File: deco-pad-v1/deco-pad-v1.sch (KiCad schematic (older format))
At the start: 84 parts, among them SW1 EC11, SW2 EC11, SW3 EC11, SW4 SW_Push, U1 ATmega32U4-MU, Y1 16MHz

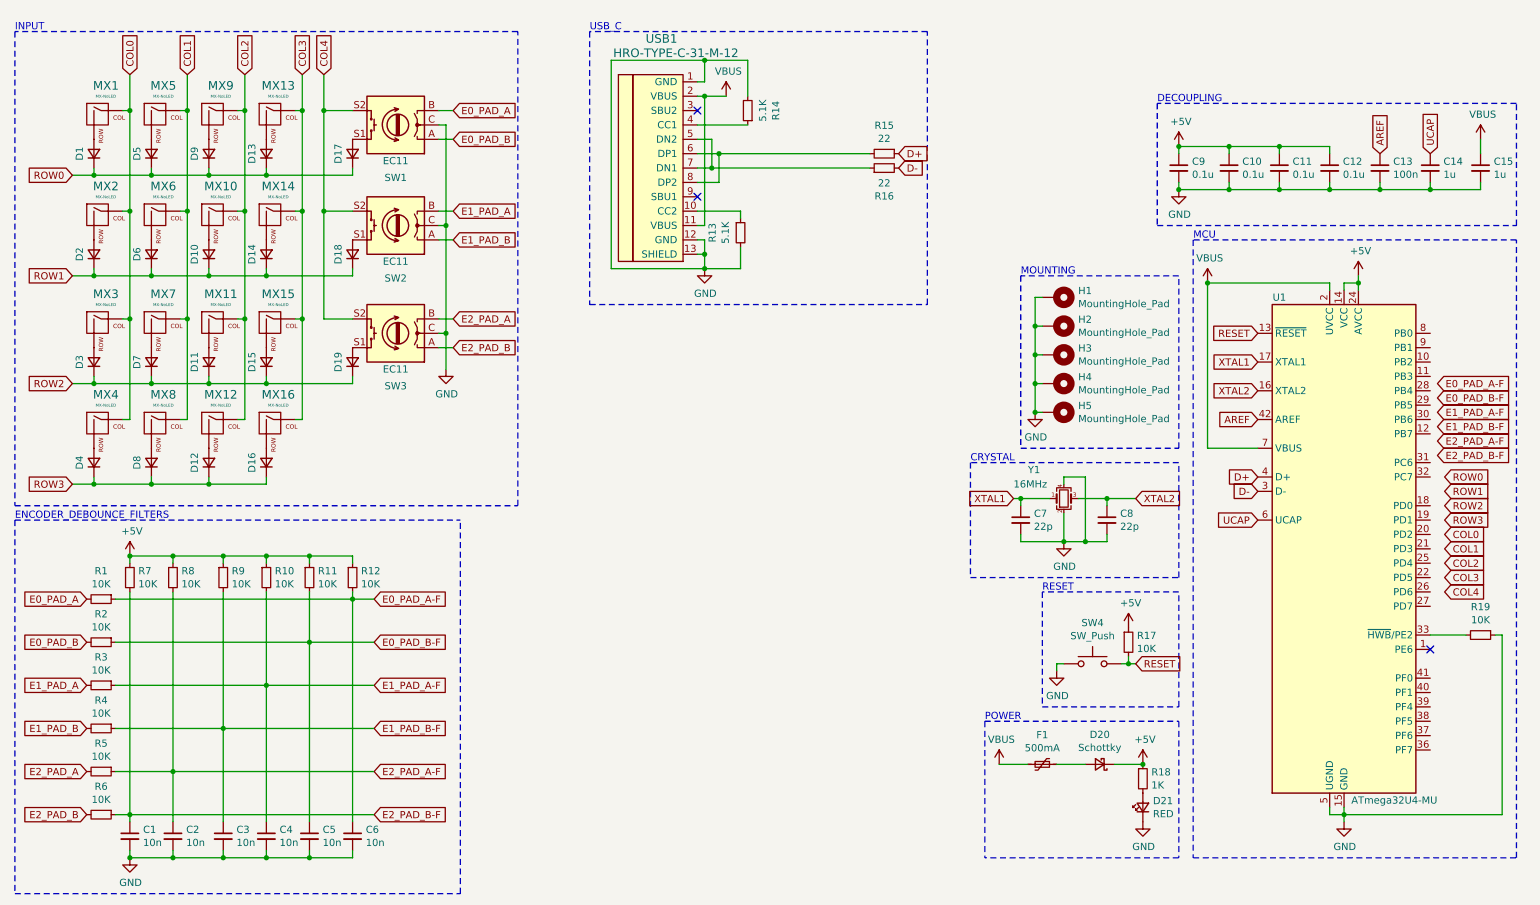
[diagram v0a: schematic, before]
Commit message: [NZ] Schematic and Footprints done.
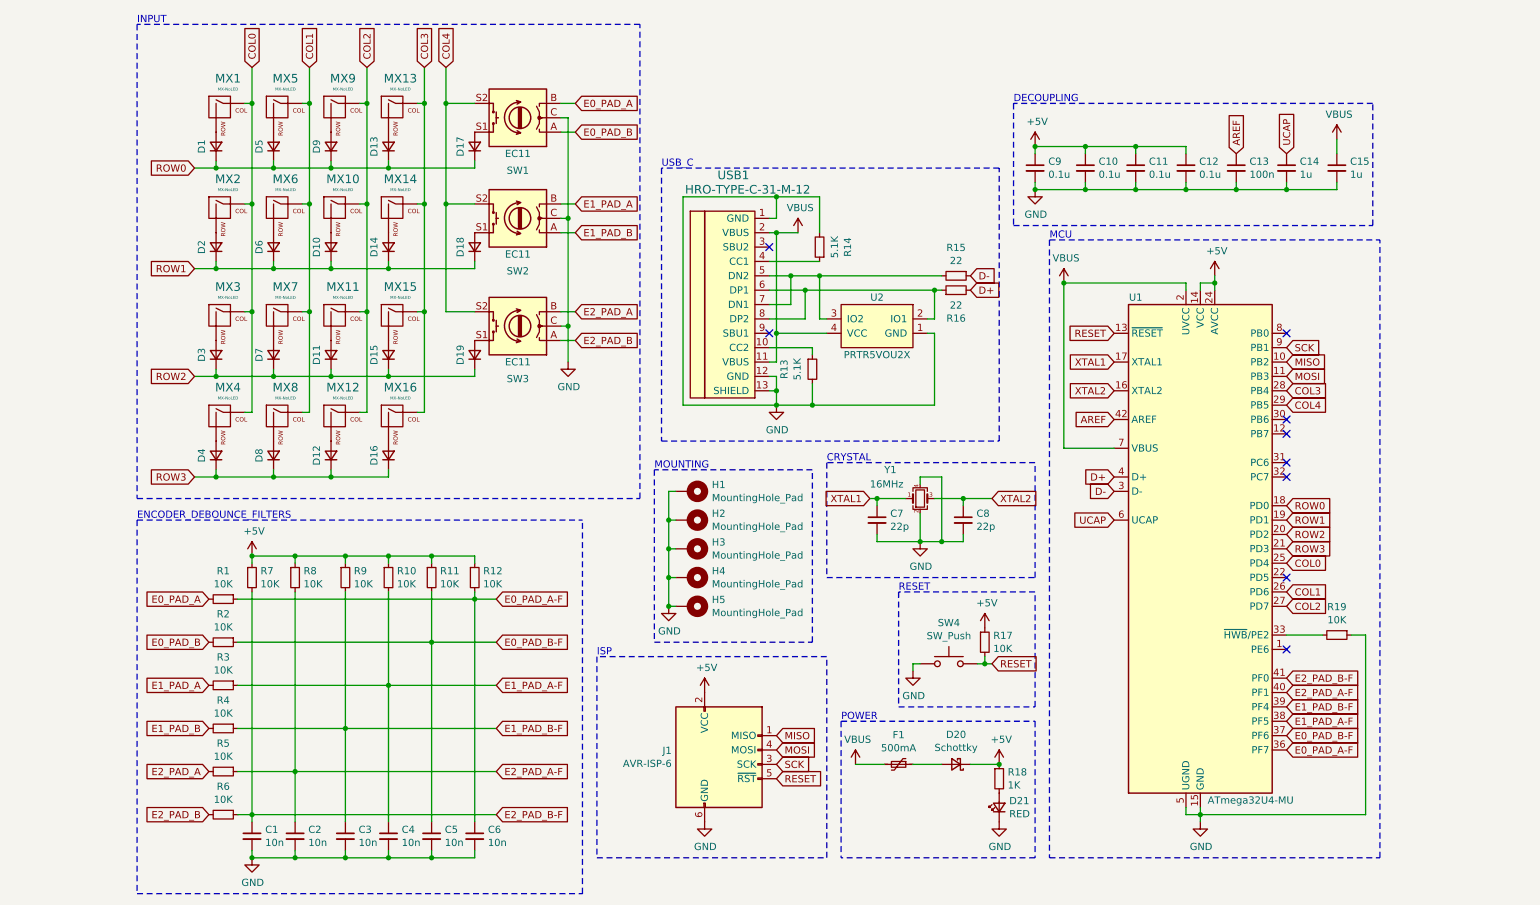
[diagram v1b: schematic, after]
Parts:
- added J1: AVR-ISP-6, Connector_PinSocket_2.54mm:PinSocket_2x03_P2.54mm_Vertical, symbol Connector:AVR-ISP-6
- added U2: PRTR5VOU2X, Nexperia:SOT143B, symbol prtr5vou2x:PRTR5VOU2X
- C1, C10, C11, C12, C13, C14, C2, C3, C4, C5, C6, C7, C8, C9: footprint Capacitor_SMD:C_0603_1608Metric -> Capacitor_SMD:C_0805_2012Metric
- D1, D10, D11, D12, D13, D14, D15, D16, D17, D18, D19, D2, D20, D3, D4, D5, D6, D7, D8, D9: footprint (none) -> Diode_SMD:D_SOD-123
- D21: footprint (none) -> LED_SMD:LED_0805_2012Metric
- F1: footprint (none) -> Fuse:Fuse_1206_3216Metric
- MX1, MX10, MX11, MX12, MX13, MX14, MX15, MX16, MX2, MX3, MX4, MX5, MX6, MX7, MX8, MX9: footprint (none) -> mx-alps-hybrid:MX-1U-NoLED
- R1, R10, R11, R12, R13, R14, R15, R16, R17, R18, R19, R2, R3, R4, R5, R6, R7, R8, R9: footprint (none) -> Resistor_SMD:R_0805_2012Metric
- SW1, SW2, SW3: footprint (none) -> Rotary_Encoder:RotaryEncoder_Alps_EC11E-Switch_Vertical_H20mm
- SW4: footprint (none) -> Button_Switch_SMD:SW_SPST_B3S-1000
- Y1: footprint (none) -> Crystal:Crystal_SMD_3225-4Pin_3.2x2.5mm
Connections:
- net +5V: now also J1.2 (VCC)
- net COL0: now also U1.25 (PD4)
- net COL1: now also U1.26 (PD6)
- net COL2: now also U1.27 (PD7)
- net COL3: now also U1.28 (PB4)
- net COL4: now also U1.29 (PB5)
- net D+: now also R16.2; no longer R15.1
- net D-: now also R15.1; no longer R16.2
- net E0_PAD_A-F: now also U1.36 (PF7)
- net E0_PAD_B-F: now also U1.37 (PF6)
- net E1_PAD_A-F: now also U1.38 (PF5)
- net E1_PAD_B-F: now also U1.39 (PF4)
- net E2_PAD_A-F: now also U1.40 (PF1)
- net E2_PAD_B-F: now also U1.41 (PF0)
- net GND: now also J1.6 (GND), U2.1 (GND)
- net RESET: now also J1.5 (~RST)
- net ROW0: now also U1.18 (PD0)
- net ROW1: now also U1.19 (PD1)
- net ROW2: now also U1.20 (PD2)
- net ROW3: now also U1.21 (PD3)
- net VBUS: now also U2.4 (VCC)
- net MISO: now reaches U1.10 (PB2)
- net MISO: now also J1.1 (MISO)
- net MOSI: now reaches U1.11 (PB3)
- net MOSI: now also J1.4 (MOSI)
- net SCK: now reaches U1.9 (PB1)
- net SCK: now also J1.3 (SCK)
- net at USB1.5 (DN2), USB1.7 (DN1): now also R15.2, U2.3 (IO2); no longer R16.1
- net at USB1.6 (DP1), USB1.8 (DP2): now also R16.1, U2.2 (IO1); no longer R15.2
- no-connect marks 3 -> 9
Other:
- note added: "ISP"
- moved on the sheet: C1, C10, C11, C12, C13, C14, C15, C2, C3, C4, C5, C6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
